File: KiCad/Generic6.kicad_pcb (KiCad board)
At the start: 2 copper layers, 18.3 x 13.5 mm, 19 parts, among them J1 Shelly, J2 A, J3 B, U1 ESP32-PICO-MINI-02, U2 LMR16006+FB

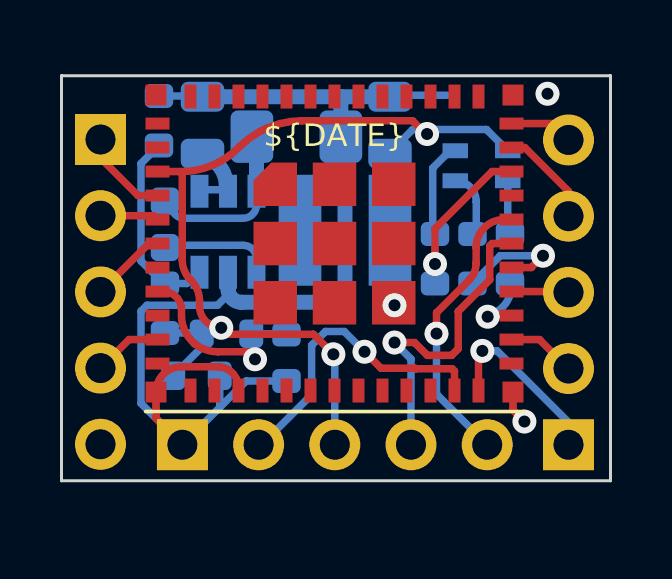
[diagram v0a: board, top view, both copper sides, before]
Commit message: Generic 6 tracked
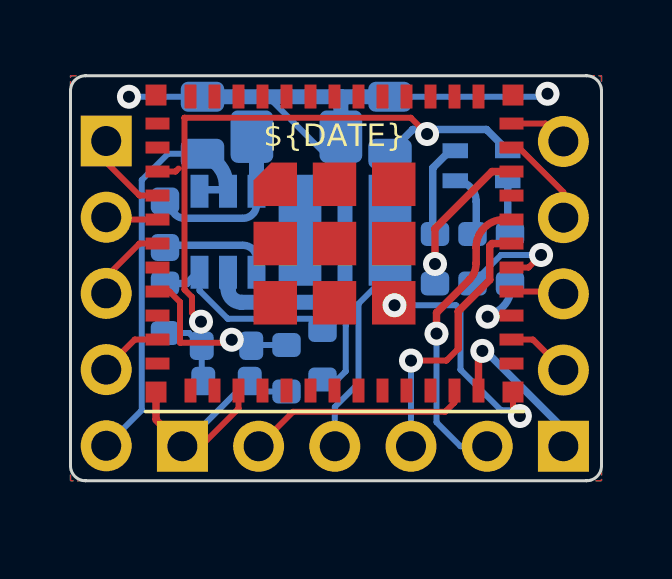
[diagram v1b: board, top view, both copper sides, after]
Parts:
- moved R6 9.52 mm to (99.6, 47.9), turned to 90 degrees
- moved C5 1.02 mm to (96.4, 48.8)
- moved R4 0.40 mm to (96.4, 47.6)
- moved C1 0.35 mm to (98.4, 48.4)
- moved J2 0.20 mm to (92.4, 40.8)
- moved J3 0.18 mm to (107.6, 51.0)
- moved J1 0.05 mm to (100.0, 51.0)
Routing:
- net GND: track 24.6 -> 38.7 mm, vias 3 -> 4
- net DC: track 0.95 -> 12.7 mm
- net GPIO0: track 10.3 -> 7.53 mm, vias 1 -> 0
- net RX: track 10.7 -> 9.22 mm
- net +3V3: track 30.7 -> 32.0 mm, vias 3 -> 2
- net TX: track 9.46 -> 10.0 mm
- net EN: track 6.44 -> 5.94 mm
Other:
- board size 18.3 x 13.5 mm -> 17.7 x 13.5 mm
- board text added: "${DATE}"
- board text added: "19/5/7"
- board text added: "20"
- board text added: "21"
- board text added: "22"
- board text added: "35"
- board text added: "36"
- board text added: "37"
- board text added: "38"
- board text added: "4"
- board text added: "8"
- board text added: "DC"
- board text added: "Generic6"
- board text removed: "22/19/7"

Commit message: Curvy tracks
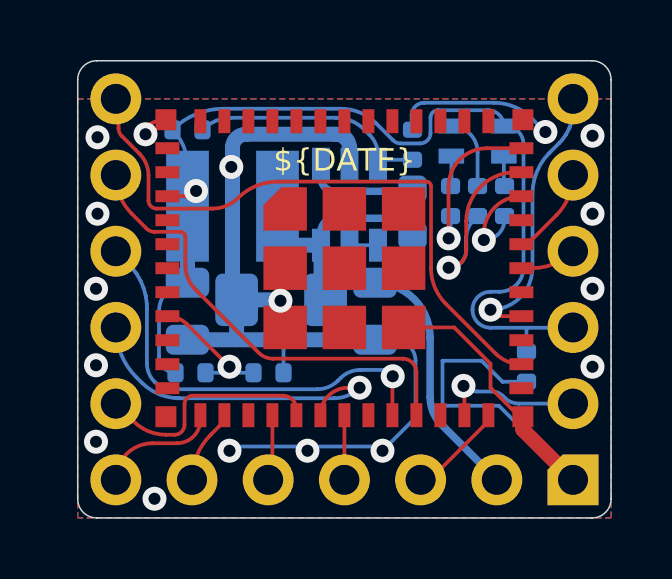
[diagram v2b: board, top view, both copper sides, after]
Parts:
- removed J2: A, Connector_PinHeader_2.54mm:PinHeader_1x05_P2.54mm_Vertical
- removed J3: B, Connector_PinHeader_2.54mm:PinHeader_1x05_P2.54mm_Vertical
- added P1: 4, RevK:Round, B.Cu at (102.9, 52.1)
- added P10: 37, RevK:Round, B.Cu at (92.7, 39.4)
- added P11: 36, RevK:Round, B.Cu at (92.7, 41.9)
- added P12: DC, RevK:Round, B.Cu at (105.4, 52.1)
- added P2: 32, RevK:Round, B.Cu at (92.7, 52.1)
- added P3: 13, RevK:Round, B.Cu at (92.7, 44.5)
- added P4: 25, RevK:Round, B.Cu at (97.8, 52.1)
- added P5: 26, RevK:Round, B.Cu at (92.7, 49.5)
- added P6: 33, RevK:Round, B.Cu at (95.2, 52.1)
- added P7: 8, RevK:Round, B.Cu at (108.0, 39.4)
- added P8: 27, RevK:Round, B.Cu at (92.7, 47.0)
- added P9: 14, RevK:Round, B.Cu at (100.3, 52.1)
- C1, C5: footprint RevK:C_0603 -> RevK:C_0402
- R1, R2, R3, R4, R5, R6: footprint RevK:R_0603 -> RevK:R_0402
- moved C5 10.0 mm to (106.4, 48.3), turned to -90 degrees
- moved J1 8.87 mm to (108.0, 47.0), turned to -90 degrees
- moved R6 7.62 mm to (102.6, 40.9), turned to -90 degrees
- moved R5 6.00 mm to (95.1, 40.4), turned to 0 degrees
- moved U2 4.15 mm to (100.5, 42.9), turned to 180 degrees
- moved R1 2.39 mm to (104.8, 42.8)
- moved R2 2.06 mm to (103.9, 42.8)
- moved R3 1.93 mm to (105.7, 42.8)
- moved R4 1.50 mm to (95.2, 48.5)
- moved U1 0.89 mm to (100.3, 45.0)
- moved D1 0.83 mm to (104.8, 40.8)
- moved C1 0.62 mm to (97.8, 48.5), turned to 180 degrees
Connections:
- net DC renamed Net-(P12-Pad1)
- net GPIO0 renamed Net-(J1-Pad2)
- net RX renamed Net-(J1-Pad4)
- net TX renamed Net-(J1-Pad5)
- U1 pad 10: IO9 -> unconnected-(U1-Pad10)
- U1 pad 12: unconnected-(U1-Pad12) -> Net-(P2-Pad1)
- U1 pad 13: unconnected-(U1-Pad13) -> Net-(P6-Pad1)
- U1 pad 15: unconnected-(U1-Pad15) -> Net-(P4-Pad1)
- U1 pad 16: unconnected-(U1-Pad16) -> Net-(P5-Pad1)
- U1 pad 17: unconnected-(U1-Pad17) -> Net-(P8-Pad1)
- U1 pad 18: unconnected-(U1-Pad18) -> Net-(P9-Pad1)
- U1 pad 20: unconnected-(U1-Pad20) -> Net-(P3-Pad1)
- U1 pad 21: unconnected-(U1-Pad21) -> Net-(U1-Pad21)
- U1 pad 24: IO1 -> Net-(P1-Pad1)
- U1 pad 26: IO2 -> Net-(U1-Pad26)
- U1 pad 27: B -> unconnected-(U1-Pad27)
- U1 pad 28: IO3 -> Net-(P7-Pad1)
- U1 pad 29: G -> unconnected-(U1-Pad29)
- U1 pad 33: R -> B
- U1 pad 34: IO4 -> R
- U1 pad 35: IO5 -> G
- U1 pad 4: IO6 -> unconnected-(U1-Pad4)
- U1 pad 5: IO7 -> unconnected-(U1-Pad5)
- U1 pad 6: IO8 -> unconnected-(U1-Pad6)
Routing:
- net Net-(U1-Pad26): track 0.00 -> 21.0 mm
- net Net-(U1-Pad21): track 0.00 -> 15.3 mm
- net Net-(P3-Pad1): track 0.00 -> 14.3 mm, vias 0 -> 1
- net Net-(P8-Pad1): track 0.00 -> 11.5 mm, vias 0 -> 1
- net Net-(P7-Pad1): track 0.00 -> 9.63 mm, vias 0 -> 1
- net Net-(P5-Pad1): track 0.00 -> 7.83 mm
- net Net-(J1-Pad4): track 9.22 -> 1.86 mm, vias 1 -> 0
- net Net-(J1-Pad5): track 10.0 -> 3.04 mm, vias 1 -> 0
- net IO1: track 5.68 -> 0.00 mm, vias 1 -> 0
- net Net-(P2-Pad1): track 0.00 -> 4.04 mm
- net Net-(P12-Pad1): track 12.7 -> 9.35 mm
- net Net-(P1-Pad1): track 0.00 -> 3.23 mm
- net IO4: track 3.20 -> 0.00 mm
- net IO6: track 2.93 -> 0.00 mm
- net Net-(J1-Pad2): track 7.53 -> 4.80 mm, vias 0 -> 1
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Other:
- board size 17.7 x 13.5 mm -> 17.8 x 15.2 mm
- board text added: "RGB: 22/21/19"
- board text removed: "19/5/7"
- board text removed: "20"
- board text removed: "21"
- board text removed: "22"
- board text removed: "35"
- board text removed: "36"
- board text removed: "37"
- board text removed: "38"
- board text removed: "4"
- board text removed: "8"
- board text removed: "DC"
